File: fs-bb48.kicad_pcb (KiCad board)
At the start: 2 copper layers, 35 x 12.1 mm, 15 parts, among them P1 USB, P2 SWD, P3 PWR, P4 EXT, T1 TOUCH_PAD, U1 MKL27Z256VFM4, U2 EMIF02-USB03F2

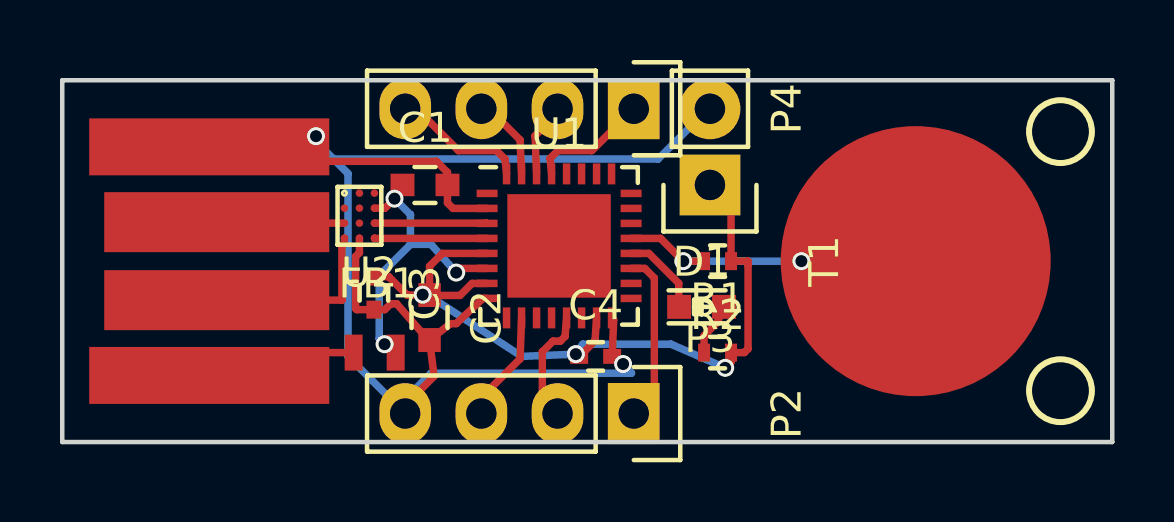
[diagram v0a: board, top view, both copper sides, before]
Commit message: update
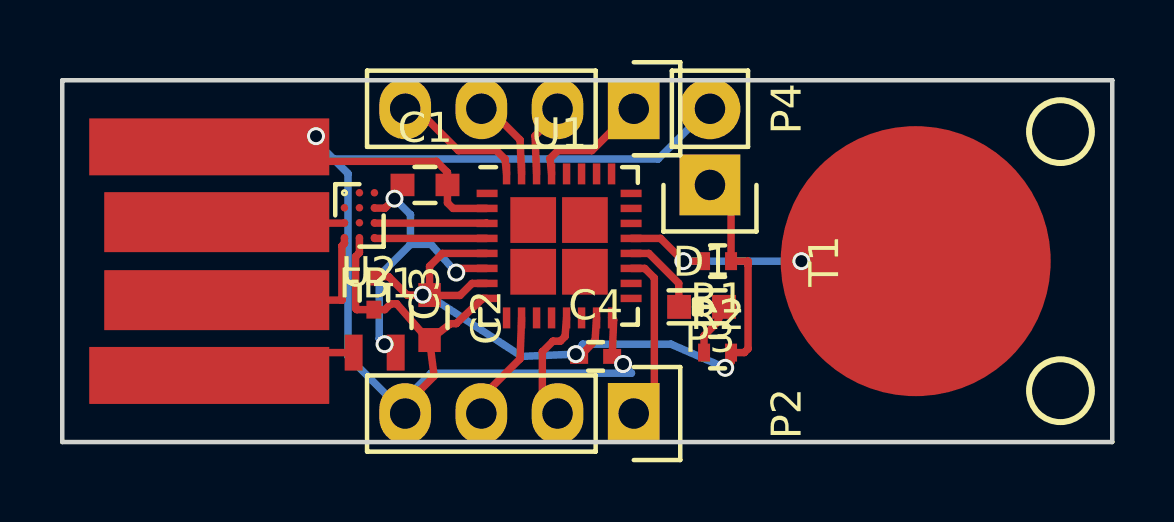
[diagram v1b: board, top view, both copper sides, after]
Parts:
- U1: footprint Housings_DFN_QFN:QFN-32-1EP_5x5mm_Pitch0.5mm -> fs-bb48:QFN-32-1EP_5x5mm_Pitch0.5mm
- moved U2 0.46 mm to (136.4, 105.4)
